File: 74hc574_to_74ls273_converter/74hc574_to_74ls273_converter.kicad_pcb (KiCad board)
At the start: 2 copper layers, 10 parts, among them J1 Conn_01x01_Pin, J2 Conn_01x01_Pin, J3 Conn_01x01_Pin, J4 Conn_01x01_Pin, J5 Conn_01x01_Pin, J6 Conn_01x01_Pin, J7 Conn_01x01_Pin, J8 Conn_01x01_Pin, U1 74LS574, U2 74LS273

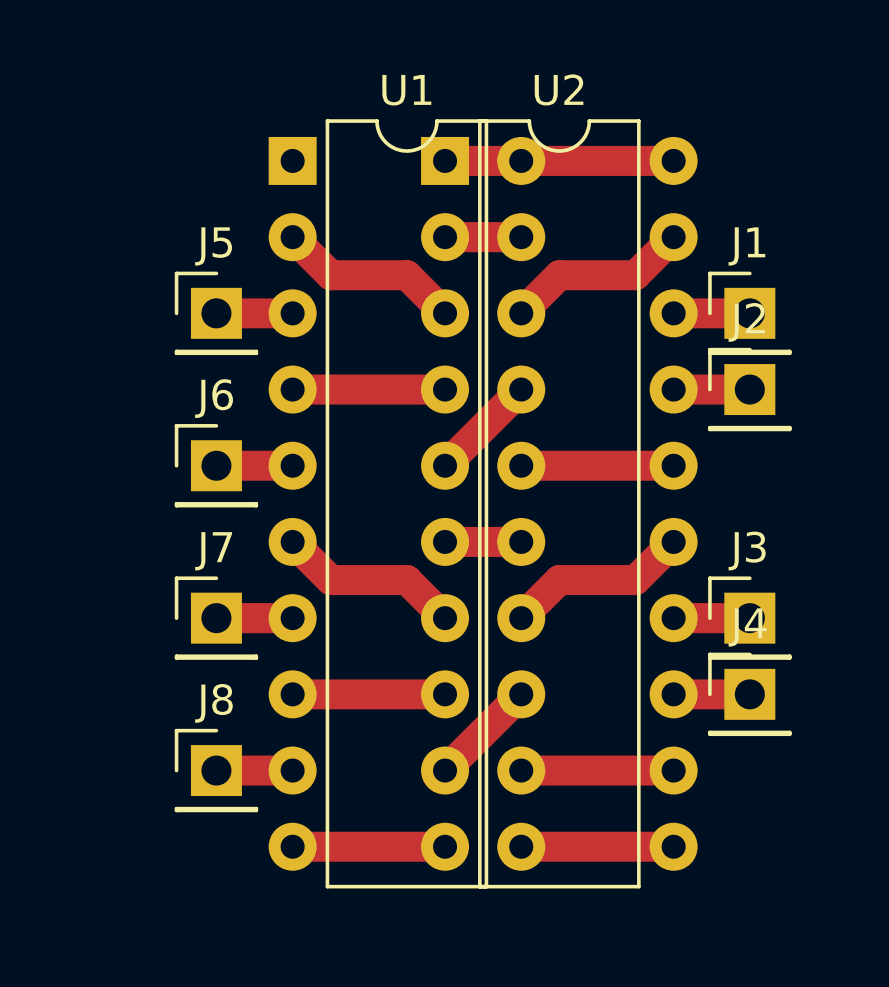
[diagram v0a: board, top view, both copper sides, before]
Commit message: test cnc
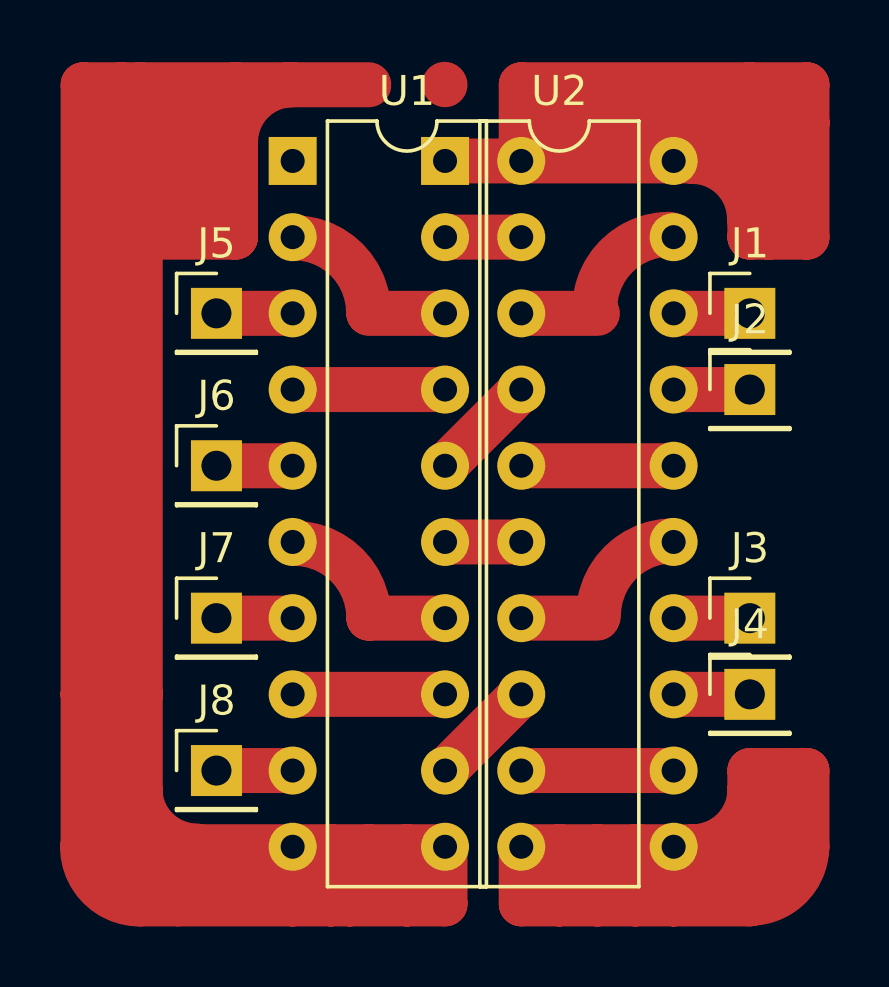
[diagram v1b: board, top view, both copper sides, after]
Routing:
- net GND: track 5.08 -> 145.9 mm
- net +5V: track 7.62 -> 46.6 mm
- net /CLK: track 5.08 -> 40.9 mm
- net /d4: track 6.13 -> 0.00 mm
- net /d0: track 6.13 -> 0.00 mm
- net /q5: track 6.13 -> 0.00 mm
- net /q1: track 6.13 -> 0.00 mm

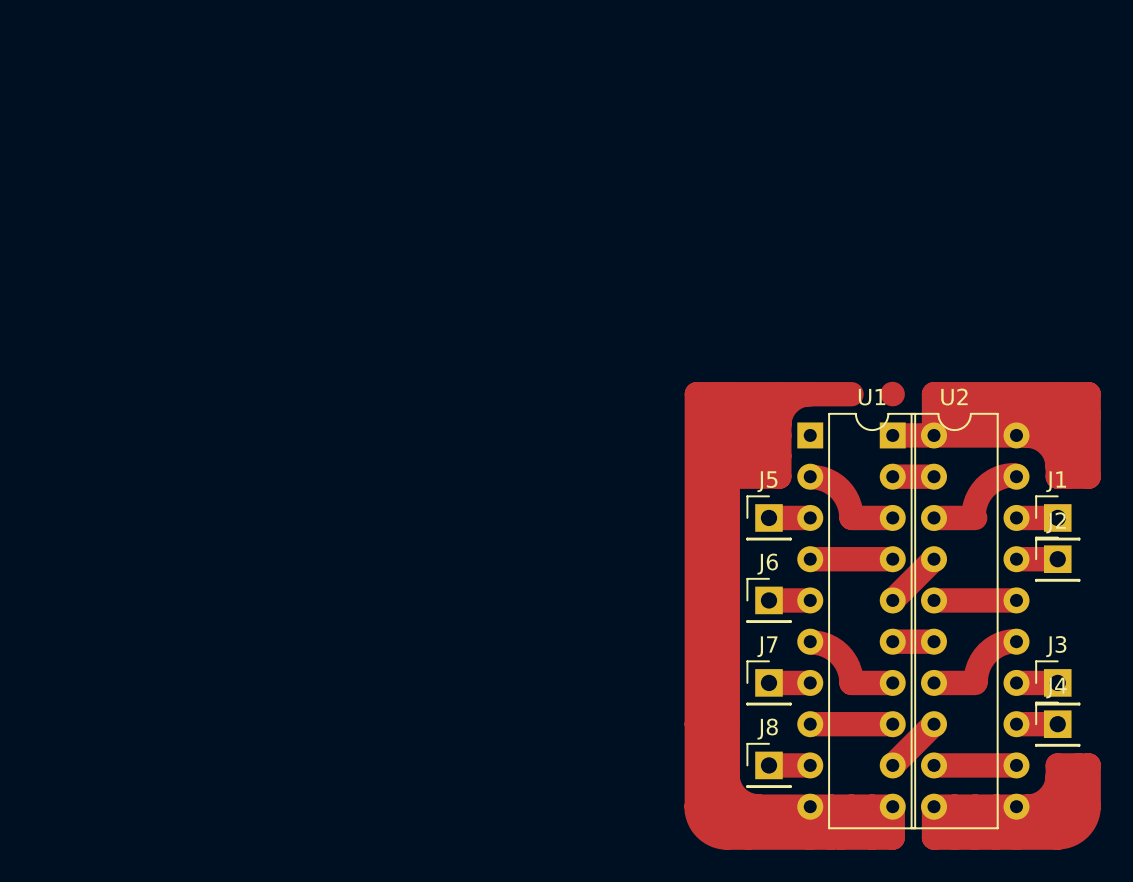
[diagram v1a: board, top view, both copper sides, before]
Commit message: YOSKRIBBA
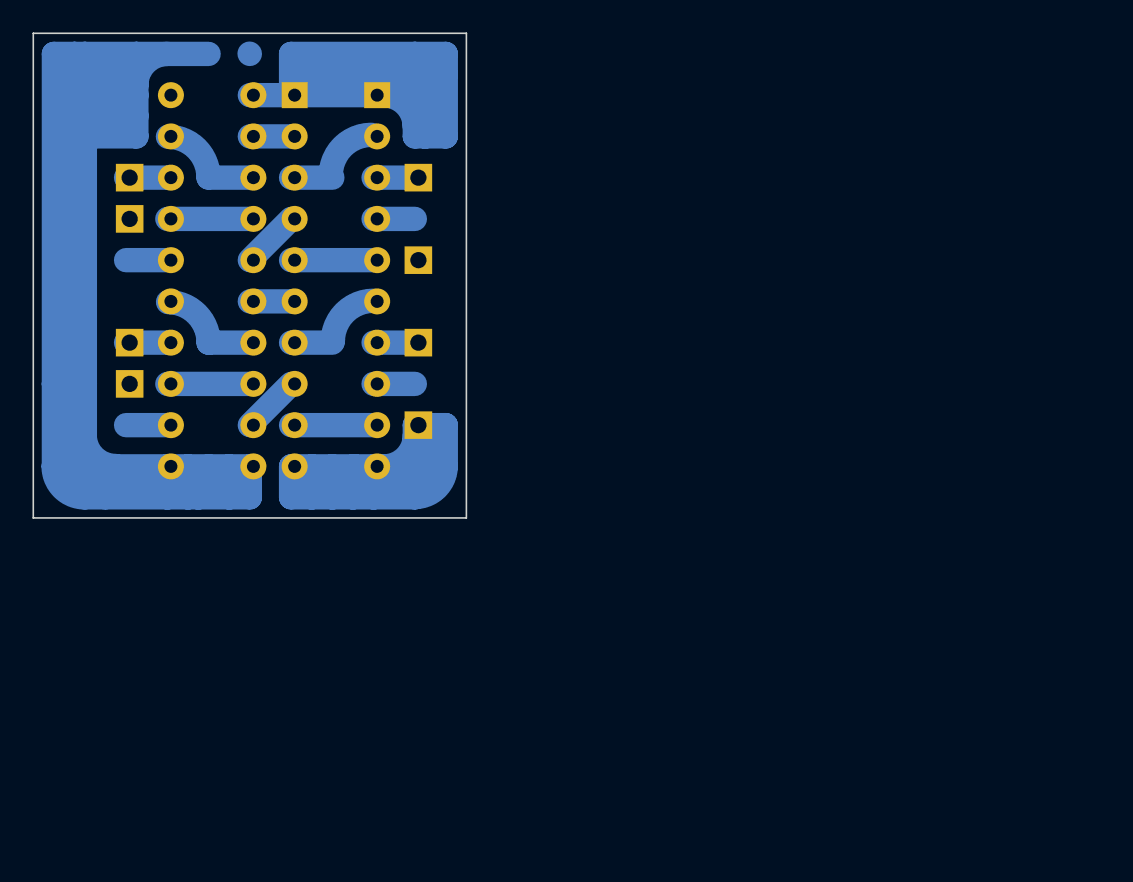
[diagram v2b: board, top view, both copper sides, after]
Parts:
- J1, J2, J3, J4, J5, J6, J7, J8, U1, U2: moved to B.Cu
- moved J1 60.9 mm to (6.35, 9.53), turned to 180 degrees
- moved J2 60.9 mm to (6.35, 12.1), turned to 180 degrees
- moved J3 60.9 mm to (6.35, 19.7), turned to 180 degrees
- moved J4 60.9 mm to (6.35, 22.2), turned to 180 degrees
- moved U2 42.4 mm to (16.5, 4.45), turned to 180 degrees
- moved U1 33.9 mm to (21.6, 4.45), turned to 180 degrees
- moved J5 30.1 mm to (24.1, 9.53), turned to 180 degrees
- moved J6 30.1 mm to (24.1, 14.6), turned to 180 degrees
- moved J7 30.1 mm to (24.1, 19.7), turned to 180 degrees
- moved J8 30.1 mm to (24.1, 24.8), turned to 180 degrees
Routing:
- net /CLK: track 40.9 -> 186.8 mm
- net GND: track 145.9 -> 0.00 mm
- net /d7: track 5.08 -> 0.00 mm
- net /d3: track 5.08 -> 0.00 mm
- net /q7: track 5.08 -> 7.62 mm
- net /q3: track 5.08 -> 7.62 mm
- net /d6: track 5.08 -> 7.62 mm
- net /d2: track 5.08 -> 7.62 mm
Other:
- board outline added: 26.7 x 29.8 mm

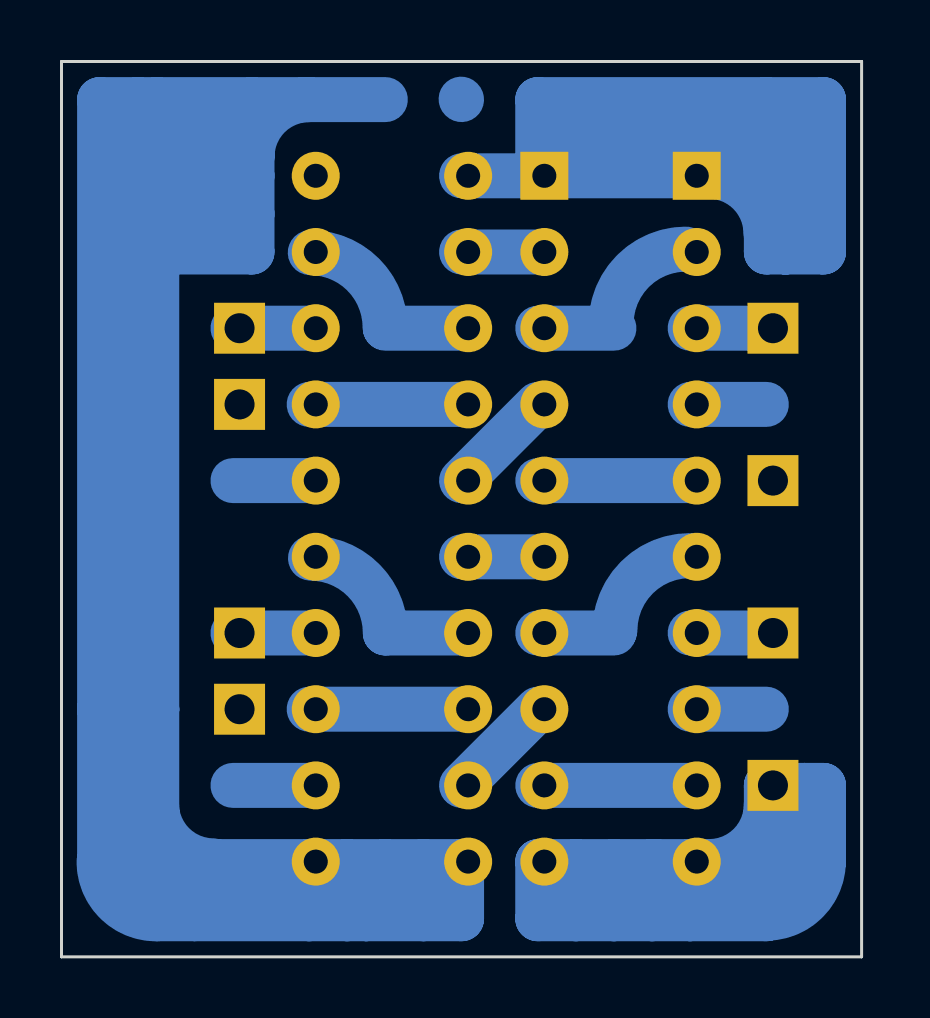
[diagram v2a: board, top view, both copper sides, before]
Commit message: psunoig
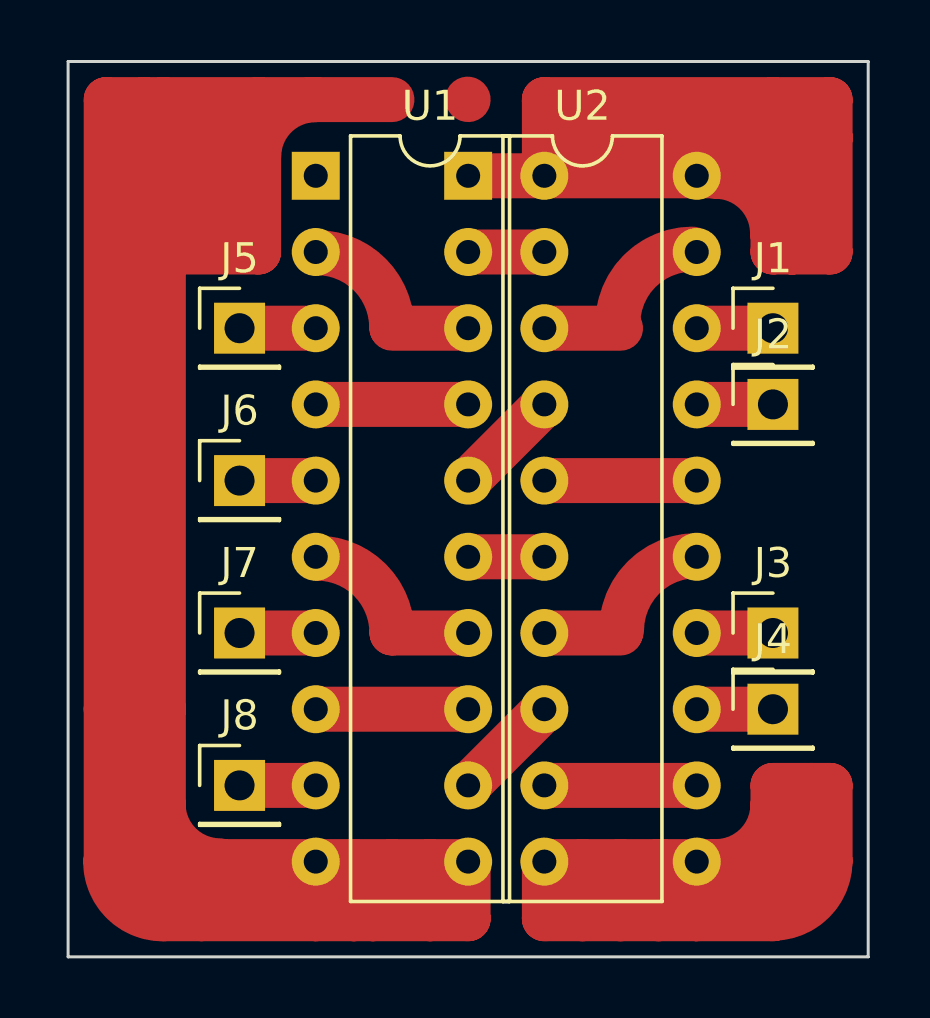
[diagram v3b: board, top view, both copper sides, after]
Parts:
- J1, J2, J3, J4, J5, J6, J7, J8, U1, U2: moved to F.Cu
- moved J1 17.8 mm to (24.1, 9.53), turned to 0 degrees
- moved J2 17.8 mm to (24.1, 12.1), turned to 0 degrees
- moved J3 17.8 mm to (24.1, 19.7), turned to 0 degrees
- moved J4 17.8 mm to (24.1, 22.2), turned to 0 degrees
- moved J5 17.8 mm to (6.35, 9.53), turned to 0 degrees
- moved J6 17.8 mm to (6.35, 14.6), turned to 0 degrees
- moved J7 17.8 mm to (6.35, 19.7), turned to 0 degrees
- moved J8 17.8 mm to (6.35, 24.8), turned to 0 degrees
- moved U1 12.7 mm to (8.89, 4.45), turned to 0 degrees
- moved U2 2.54 mm to (14.0, 4.45), turned to 0 degrees
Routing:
- net /CLK: track 186.8 -> 40.9 mm
- net GND: track 0.00 -> 145.9 mm
- net /d7: track 0.00 -> 5.08 mm
- net /d3: track 0.00 -> 5.08 mm
- net /q7: track 7.62 -> 5.08 mm
- net /q3: track 7.62 -> 5.08 mm
- net /d6: track 7.62 -> 5.08 mm
- net /d2: track 7.62 -> 5.08 mm
